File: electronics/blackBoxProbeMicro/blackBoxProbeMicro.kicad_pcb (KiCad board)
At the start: 4 copper layers, 29 x 29 mm, 60 parts, among them J1 USB-C, J2 JTAG_2X05, J3 JTAG_2X05, J4 DevBoardUartOutput, Q1 Q_NMOS_DUAL, Q2 Q_PMOS_DUAL, U1 MCP1702-MB, U2 USBLC6-2, U3 STM32F103CBT, Y1 8MHz

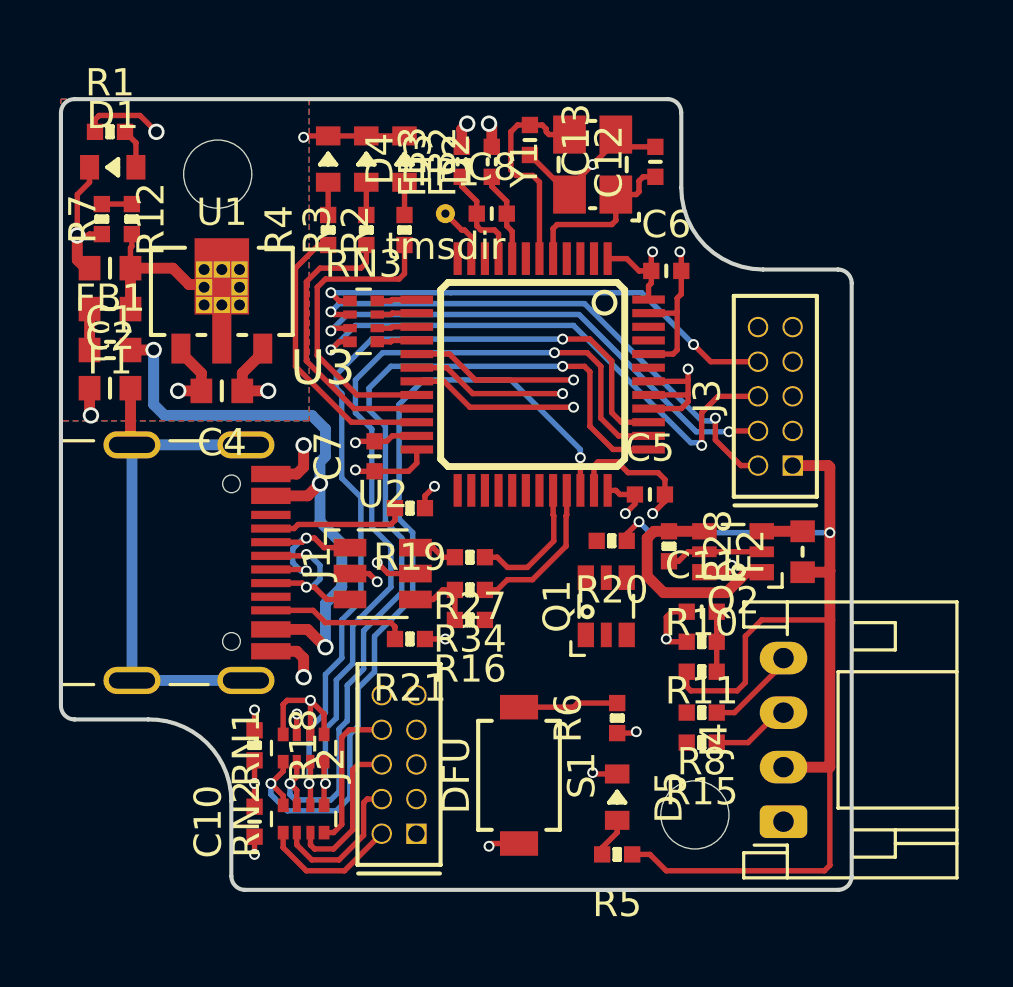
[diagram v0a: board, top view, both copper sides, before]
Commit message: further routing
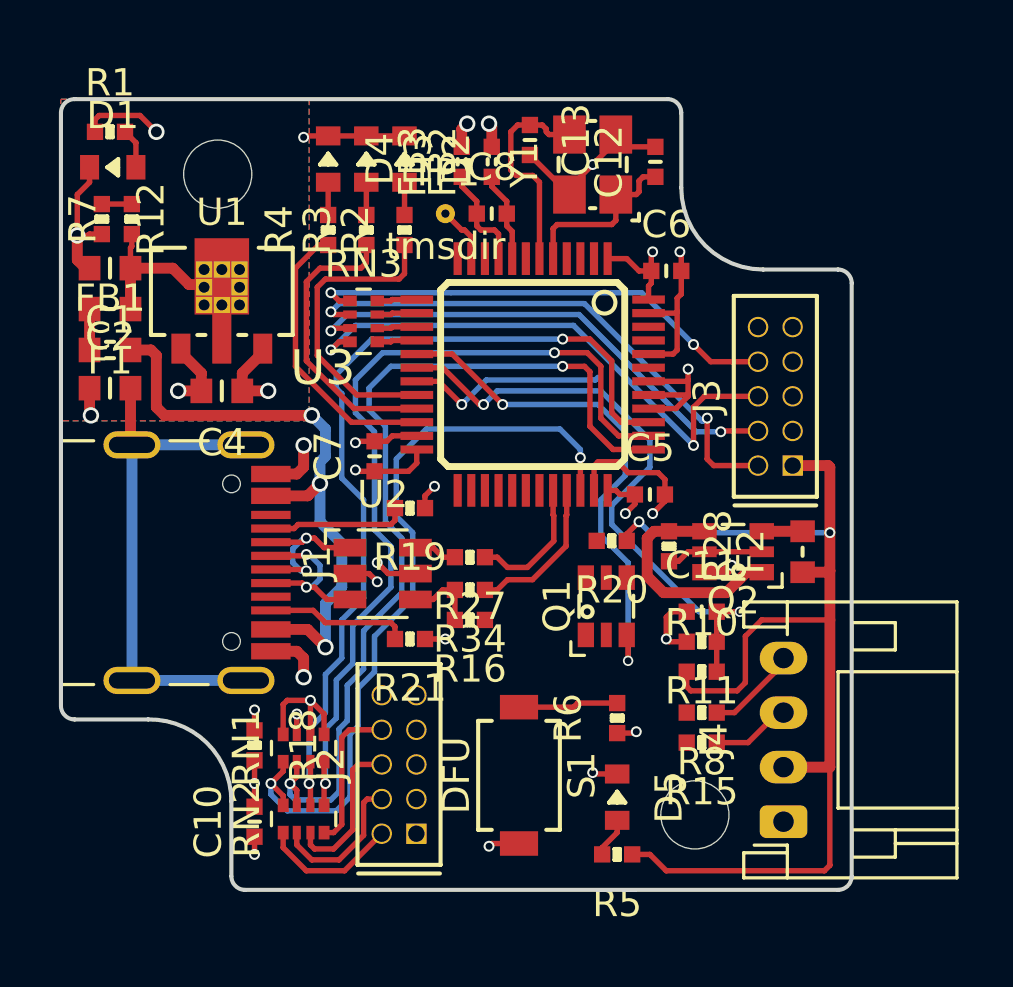
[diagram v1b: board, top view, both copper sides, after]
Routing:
- net /TARGET_PWR_SENSE: track 7.94 -> 22.8 mm, vias 1 -> 2
- net /PROBE_I_RST_SEN: track 6.14 -> 19.0 mm, vias 1 -> 2
- net /MCU_TMS: track 30.8 -> 28.2 mm
- net /TARGET_PWR_EN: track 9.69 -> 11.0 mm
